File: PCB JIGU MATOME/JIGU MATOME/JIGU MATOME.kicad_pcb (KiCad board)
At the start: 2 copper layers, 7 parts, among them J1 Conn_01x04, J2 Conn_01x04, J3 Conn_01x04, J4 Conn_01x04, J5 Conn_01x08, J6 Conn_01x06, U1 757BS

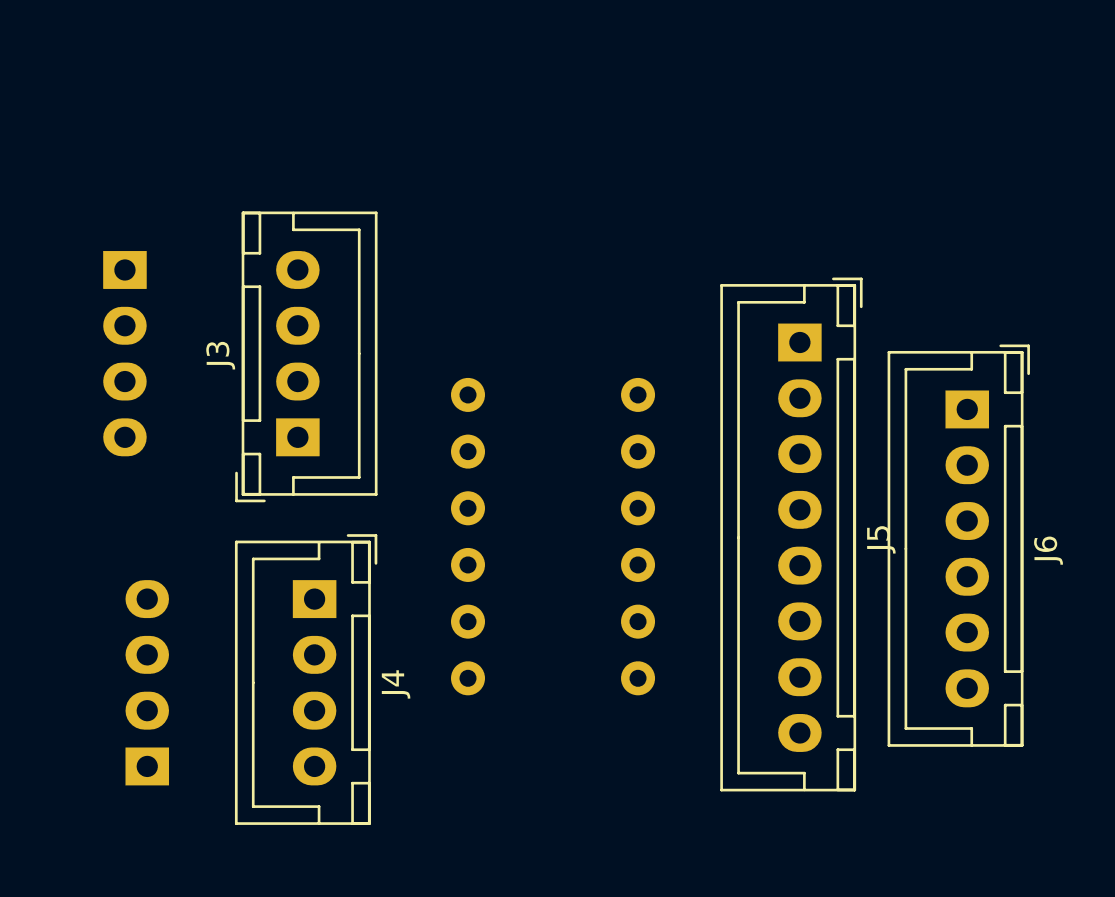
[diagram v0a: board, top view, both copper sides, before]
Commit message: modifier pcb jigu
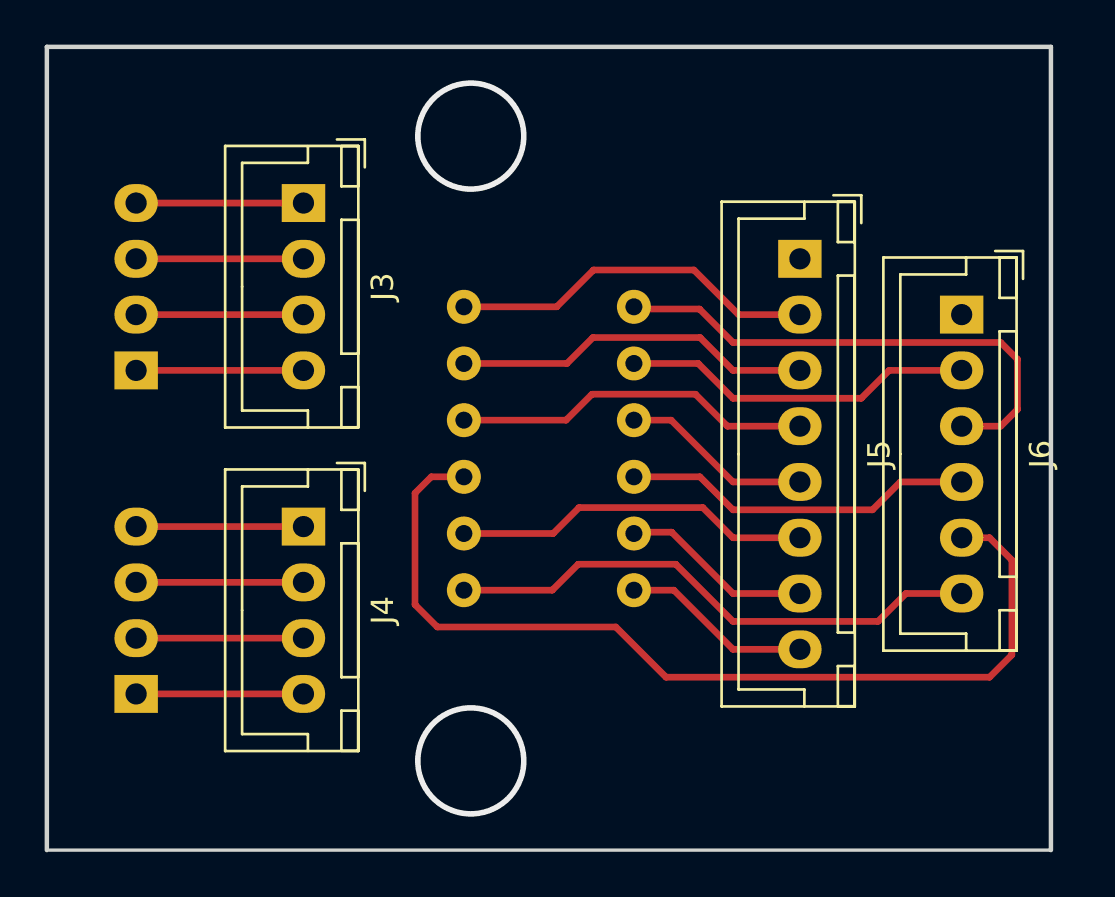
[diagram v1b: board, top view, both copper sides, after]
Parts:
- moved J3 10.5 mm to (131.2, 88.0), turned to 270 degrees
- moved J1 4.53 mm to (123.8, 95.5), turned to 90 degrees
- moved J6 4.26 mm to (160.8, 93.0)
- moved U1 3.95 mm to (142.2, 99.0)
- moved J5 3.75 mm to (153.5, 90.5)
- moved J2 3.29 mm to (123.8, 110.0)
- moved J4 3.29 mm to (131.2, 102.5)
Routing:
- net Net-(J6-Pad5): track 0.00 -> 42.9 mm
- net Net-(J6-Pad6): track 0.00 -> 24.4 mm
- net Net-(J6-Pad3): track 0.00 -> 23.2 mm
- net Net-(J5-Pad2): track 0.00 -> 16.6 mm
- net Net-(J5-Pad3): track 0.00 -> 16.2 mm
- net Net-(J5-Pad4): track 0.00 -> 16.1 mm
- net Net-(J5-Pad6): track 0.00 -> 16.1 mm
- net Net-(J6-Pad2): track 0.00 -> 15.9 mm
- net Net-(J6-Pad4): track 0.00 -> 15.8 mm
- net Net-(J5-Pad7): track 0.00 -> 8.60 mm
- net Net-(J5-Pad5): track 0.00 -> 8.59 mm
- net Net-(J5-Pad8): track 0.00 -> 8.54 mm
- net Net-(J2-Pad4): track 0.00 -> 7.50 mm
- net Net-(J2-Pad3): track 0.00 -> 7.50 mm
- net Net-(J2-Pad2): track 0.00 -> 7.50 mm
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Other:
- board outline added: 45 x 36 mm
- net class SIG added: clearance 0.25, trace_width 0.3, via_dia 1, via_drill 0.5
